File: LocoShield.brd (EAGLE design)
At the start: 44.5 x 50 mm, 22 parts, among them J2 RJ12, J3 RJ12, Q1 2N3904, U1 LM393M, U2 LM317LCDR

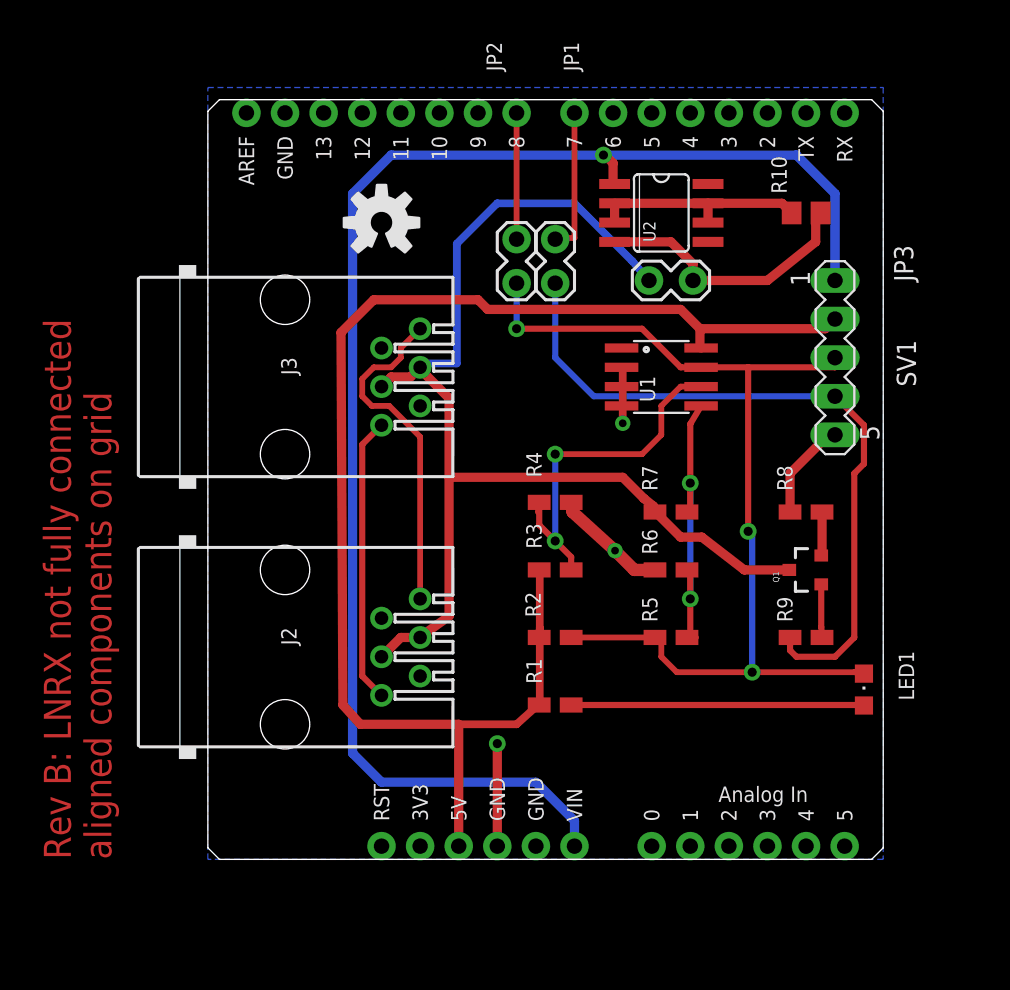
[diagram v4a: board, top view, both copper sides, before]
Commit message: 1.4
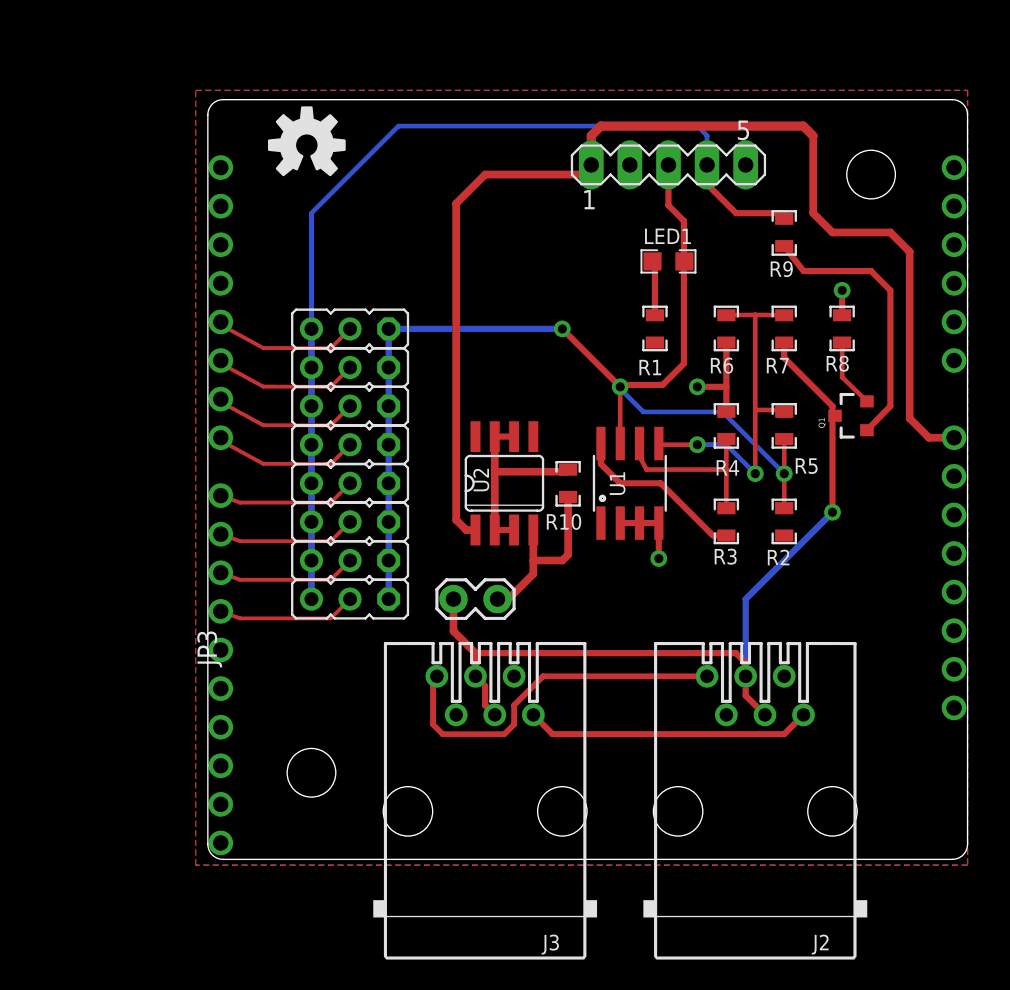
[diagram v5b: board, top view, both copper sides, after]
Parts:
- removed JP1, JP2: (no value), MCP:1X02_LOCK
- added JPD10, JPD11, JPD4, JPD5, JPD6, JPD7, JPD8, JPD9: (no value), MCP:JP2
- LED1: value (none) -> Blue; device MCP:CHIPLED_0805 -> SPCoast:0805-LED
- R1, R2, R3, R4, R5, R6, R7, R8, R9: device rcl:R0805W -> SPCoast:0805-RES
- R10: device rcl:R0805 -> SPCoast:0805-RES
- SHIELD: value ARDUINO_SHIELDNOHOLES -> ARDUINO_SHIELDNO_SILK; device SparkFun:DUEMILANOVE_SHIELD_NOHOLES -> SPCoast:DUEMILANOVE_VIAS
- moved SHIELD 53.3 mm to (-0.42, -0.19), turned to 0 degrees
- moved J2 32.8 mm to (36.0, 3.16), turned to 0 degrees
- moved J3 31.5 mm to (18.2, 3.16), turned to 0 degrees
- moved LED1 31.0 mm to (30.3, 39.4)
- moved R9 26.7 mm to (37.9, 41.3), turned to 270 degrees
- moved R1 25.6 mm to (29.4, 34.9), turned to 90 degrees
- moved JP3 24.6 mm to (16.3, 17.1)
- moved R10 23.7 mm to (23.7, 24.8), turned to 270 degrees
- moved U2 20.6 mm to (19.5, 24.8), turned to 0 degrees
- moved R2 16.9 mm to (37.9, 22.2), turned to 90 degrees
- moved SV1 16.8 mm to (30.3, 45.7), turned to 0 degrees
- moved R6 16.3 mm to (34.1, 34.9), turned to 90 degrees
- moved R5 15.8 mm to (37.9, 28.6), turned to 270 degrees
- moved R7 14.2 mm to (37.9, 34.9), turned to 90 degrees
- moved R4 12.4 mm to (34.1, 28.6), turned to 270 degrees
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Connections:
- removed net N$3: JP1.1, SHIELD.D7
- removed net N$4: JP2.1, SHIELD.D8
- new net D10: JPD10.2, SHIELD.D10
- new net D11: JPD11.2, SHIELD.D11
- new net D4: JPD4.2, SHIELD.D4
- new net D5: JPD5.2, SHIELD.D5
- new net D6: JPD6.2, SHIELD.D6
- new net D7: JPD7.2, SHIELD.D7
- new net D8: JPD8.2, SHIELD.D8
- new net D9: JPD9.2, SHIELD.D9
- net GND: now also R8.2; no longer R8.1
- net LNRX: now also JPD10.1, JPD11.1, JPD4.1, JPD5.1, JPD6.1, JPD7.1, JPD8.1, JPD9.1; no longer JP2.2
- net LNTX: now also JPD10.3, JPD11.3, JPD4.3, JPD5.3, JPD6.3, JPD7.3, JPD8.3, JPD9.3; no longer JP1.2
- net N$6: now also R8.1; no longer R8.2
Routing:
- net VCC: track 92.2 -> 11.6 mm
- net V+: track 96.8 -> 76.3 mm, vias 1 -> 0
- net LOCONET: track 76.8 -> 56.6 mm, vias 0 -> 1
- net LNTX: track 47.1 -> 64.8 mm
- net N$15: track 19.3 -> 3.61 mm
- net N$1: track 3.50 -> 18.1 mm
- net N$5: track 24.3 -> 11.6 mm, vias 2 -> 0
- net GND: track 24.8 -> 13.0 mm
- net D7: track 0.00 -> 9.61 mm
- net D6: track 0.00 -> 9.61 mm
- net D5: track 0.00 -> 9.61 mm
- net D4: track 0.00 -> 9.61 mm
- net N$3: track 9.58 -> 0.00 mm
- net D10: track 0.00 -> 9.12 mm
- net D8: track 0.00 -> 9.12 mm
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- added copper zone on layer 1, net VCC
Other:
- board size 44.5 x 50 mm -> 50 x 50 mm
- board text added: "10"
- board text added: "12v"
- board text added: "2012.03"
- board text added: "2012.08"
- board text added: "2013.05"
- board text added: "2014.07"
- board text added: "5"
- board text added: "5v"
- board text added: "6"
- board text added: "7"
- board text added: "8"
- board text added: "9"
- board text added: "D11"
- board text added: "D4"
- board text added: "D4=RX"
- board text added: "D5=TX"
- board text added: "D8=RX"
- board text added: "D9=TX"
- board text added: "LEO"
- board text added: "RX pin goes to Timer ICP pin Uno -> pin 8 Leonardo -> pin 4 Mega -> pin 48 (Timer 5) or 49 (T4)"
- board text added: "TERM"
- board text added: "UNO"
- board text added: "v1.4"
- board text removed: "12v DC"
- board text removed: "2013.05 A"
- board text removed: "2014.09 B"
- board text removed: "5v DC"
- board text removed: "BLUE"
- board text removed: "D7 = TX"
- board text removed: "D8 = RX"
- board text removed: "Rev B: LNRX not fully connected aligned components on grid"
- board text removed: "Rev. 1.3B"

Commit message: added missing values
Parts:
- J2, J3: value RJ12 -> RJ12/6
- JPD10, JPD11, JPD4, JPD5, JPD6, JPD7, JPD8, JPD9, SV1: value (none) -> 0.100
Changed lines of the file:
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@@
 </autorouter>
 <elements>
-<element name="J2" library="con-amp" package="520250-3" value="RJ12" x="36.0299" y="3.16" smashed="yes">
+<element name="J2" library="con-amp" package="520250-3" value="RJ12/6" x="36.0299" y="3.16" smashed="yes">
 <attribute name="NAME" x="40.9829" y="-4.968" size="1.016" layer="25" font="vector" rot="R180"/>
 <attribute name="VALUE" x="37.1729" y="-4.333" size="1.016" layer="27" font="vector" rot="R180"/>
 </element>
-<element name="J3" library="con-amp" package="520250-3" value="RJ12" x="18.2499" y="3.16" smashed="yes">
+<element name="J3" library="con-amp" package="520250-3" value="RJ12/6" x="18.2499" y="3.16" smashed="yes">
 <attribute name="NAME" x="23.2029" y="-4.968" size="1.016" layer="25" font="vector" rot="R180"/>
 <attribute name="VALUE" x="18.1229" y="-4.333" size="1.016" layer="27" font="vector" rot="R180"/>
@@
 <attribute name="NAME" x="18.5039" y="24.115" size="1.016" layer="25" ratio="10" rot="R90"/>
 </element>
-<element name="SV1" library="con-lstb" package="MA05-1" value="" x="30.3149" y="45.705" smashed="yes">
+<element name="SV1" library="con-lstb" package="MA05-1" value="0.100" x="30.3149" y="45.705" smashed="yes">
 <attribute name="OC_NEWARK" value="unknown" x="30.3149" y="45.705" size="0.8128" layer="27" display="off"/>
 <attribute name="MPN" value="" x="30.3149" y="45.705" size="0.8128" layer="27" display="off"/>
@@
 <attribute name="VALUE" x="27.7749" y="42.784" size="1.27" layer="27" ratio="10"/>
 </element>
-<element name="JPD7" library="MCP" package="JP2" value="" x="9.3599" y="27.29" smashed="yes" rot="R180">
+<element name="JPD7" library="MCP" package="JP2" value="0.100" x="9.3599" y="27.29" smashed="yes" rot="R180">
 <attribute name="VALUE" x="5.2959" y="27.798" size="1.27" layer="27" ratio="10" rot="R180"/>
 </element>
-<element name="JPD6" library="MCP" package="JP2" value="" x="9.3599" y="29.83" smashed="yes" rot="R180">
+<element name="JPD6" library="MCP" package="JP2" value="0.100" x="9.3599" y="29.83" smashed="yes" rot="R180">
 <attribute name="VALUE" x="5.2959" y="30.338" size="1.27" layer="27" ratio="10" rot="R180"/>
 </element>
-<element name="JPD5" library="MCP" package="JP2" value="" x="9.3599" y="32.37" smashed="yes" rot="R180">
+<element name="JPD5" library="MCP" package="JP2" value="0.100" x="9.3599" y="32.37" smashed="yes" rot="R180">
 <attribute name="VALUE" x="5.2959" y="32.878" size="1.27" layer="27" ratio="10" rot="R180"/>
 </element>
-<element name="JPD4" library="MCP" package="JP2" value="" x="9.3599" y="34.91" smashed="yes" rot="R180">
+<element name="JPD4" library="MCP" package="JP2" value="0.100" x="9.3599" y="34.91" smashed="yes" rot="R180">
 <attribute name="VALUE" x="5.2959" y="35.418" size="1.27" layer="27" ratio="10" rot="R180"/>
 </element>
-<element name="JPD8" library="MCP" package="JP2" value="" x="9.3599" y="24.75" smashed="yes" rot="R180">
+<element name="JPD8" library="MCP" package="JP2" value="0.100" x="9.3599" y="24.75" smashed="yes" rot="R180">
 <attribute name="VALUE" x="5.2959" y="25.258" size="1.27" layer="27" ratio="10" rot="R180"/>
 </element>
-<element name="JPD9" library="MCP" package="JP2" value="" x="9.3599" y="22.21" smashed="yes" rot="R180">
+<element name="JPD9" library="MCP" package="JP2" value="0.100" x="9.3599" y="22.21" smashed="yes" rot="R180">
 <attribute name="VALUE" x="5.2959" y="22.718" size="1.27" layer="27" ratio="10" rot="R180"/>
 </element>
-<element name="JPD10" library="MCP" package="JP2" value="" x="9.3599" y="19.67" smashed="yes" rot="R180">
+<element name="JPD10" library="MCP" package="JP2" value="0.100" x="9.3599" y="19.67" smashed="yes" rot="R180">
 <attribute name="VALUE" x="5.2959" y="20.178" size="1.27" layer="27" ratio="10" rot="R180"/>
 </element>
-<element name="JPD11" library="MCP" package="JP2" value="" x="9.3599" y="17.13" smashed="yes" rot="R180">
+<element name="JPD11" library="MCP" package="JP2" value="0.100" x="9.3599" y="17.13" smashed="yes" rot="R180">
 <attribute name="VALUE" x="5.2959" y="17.638" size="1.27" layer="27" ratio="10" rot="R180"/>
 </element>
